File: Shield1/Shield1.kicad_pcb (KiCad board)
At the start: 4 copper layers, 12 x 14.2 mm, 26 parts, among them J1 Conn_01x01_Male, J10 Conn_01x01_Male, J11 Conn_01x01_Male, J12 Conn_01x01_Male, J13 Conn_01x01_Male, J14 Conn_01x01_Male, J15 Conn_01x01_Male, J17 Conn_01x01_Male, J2 Conn_01x01_Male, J25 Conn_01x01_Male, J26 Conn_01x01_Male, J27 Conn_01x01_Male, J28 Conn_01x01_Male, J29 Conn_01x01_Male, J3 Conn_01x01_Male, J5 Conn_01x01_Male, J6 Conn_01x01_Male, J7 Conn_01x01_Male, J8 Conn_01x01_Male, J9 Conn_01x01_Male, X1 USB_C_24pins

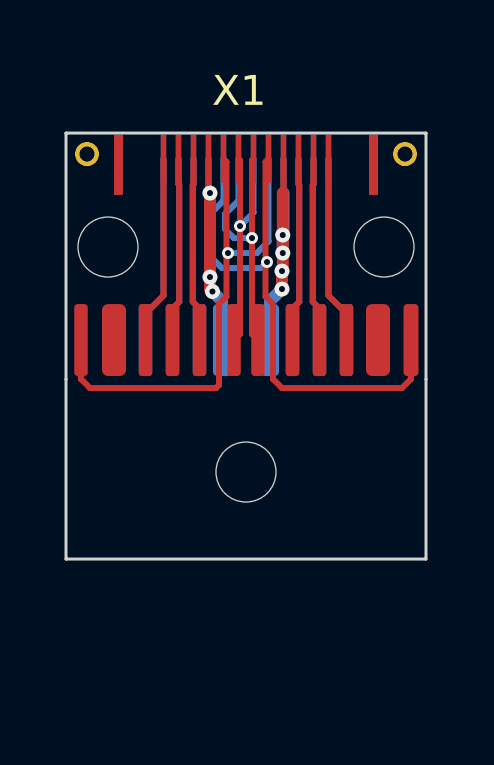
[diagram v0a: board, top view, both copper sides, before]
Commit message: v0.95 need 4 checkup
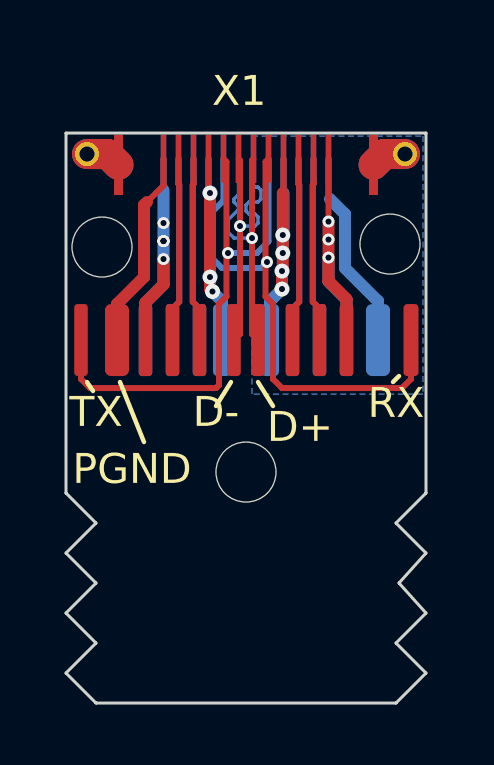
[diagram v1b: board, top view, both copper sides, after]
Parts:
- ?: moved to B.Cu
- moved ? 0.22 mm to (104.8, 23.8)
- moved ? 0.20 mm to (95.2, 23.8)
- moved ? 0.10 mm to (95.7, 26.9)
- turned ? to 180 degrees
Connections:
- ? pad 1: GND1 -> GND3
- ? pad 1: GND2 -> GND
- X1 pad 0: (no net) -> Earth
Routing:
- net GND: track 0.00 -> 6.72 mm
- net Earth: track 0.00 -> 4.80 mm
- net GND1: track 6.29 -> 9.24 mm, vias 0 -> 4
- net GND2: track 12.6 -> 9.89 mm, vias 0 -> 3
- net D-: track 8.57 -> 9.74 mm
- added copper zone on In1.Cu, net GND1
- added copper zone on In2.Cu, net GND1
- added copper zone on B.Cu, net GND2
- added copper zone on In1.Cu, net GND2
- added copper zone on In2.Cu, net GND2
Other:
- board size 12 x 14.2 mm -> 12 x 19 mm
- board text added: "D+"
- board text added: "D-"
- board text added: "PGND"
- board text added: "RX"
- board text added: "TX"
- board text added: "V1"
- board text added: "V2"
